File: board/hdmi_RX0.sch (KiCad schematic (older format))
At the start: 21 parts

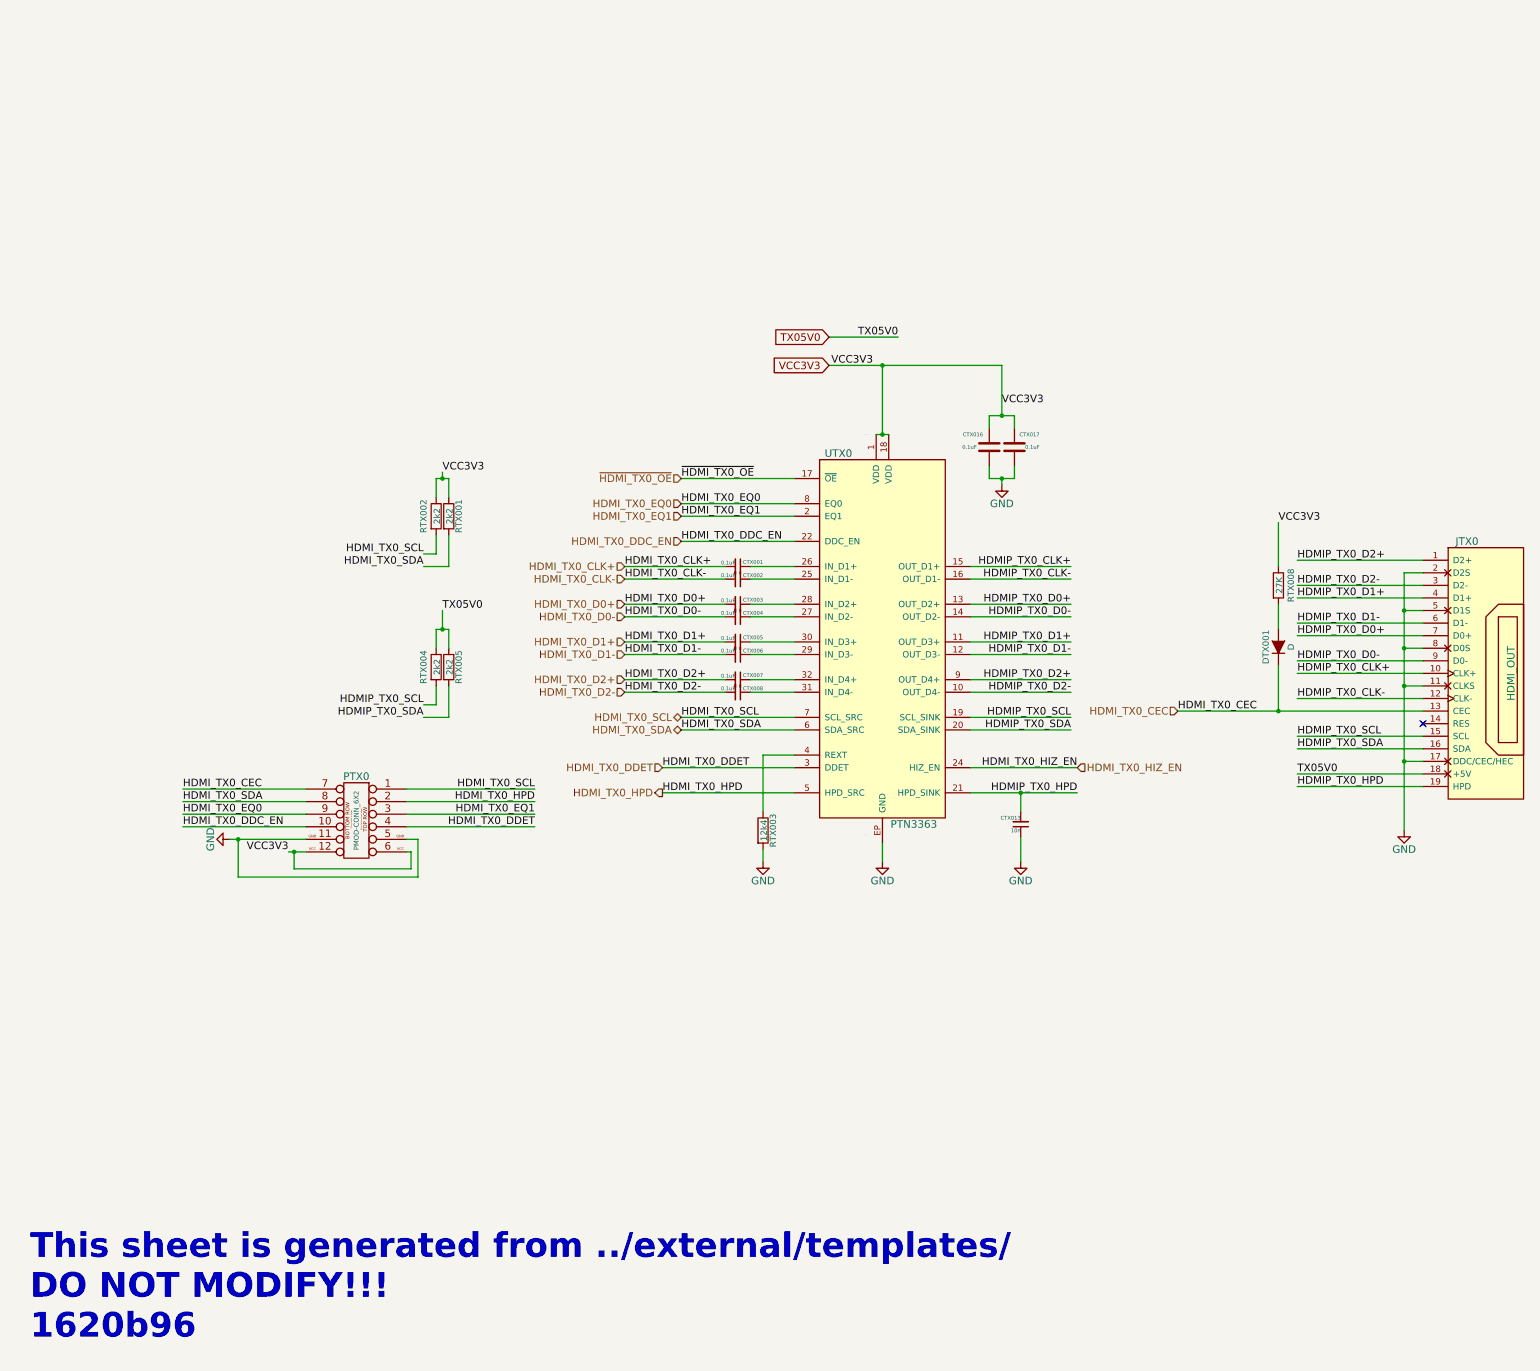
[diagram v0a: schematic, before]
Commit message: Updating from template.
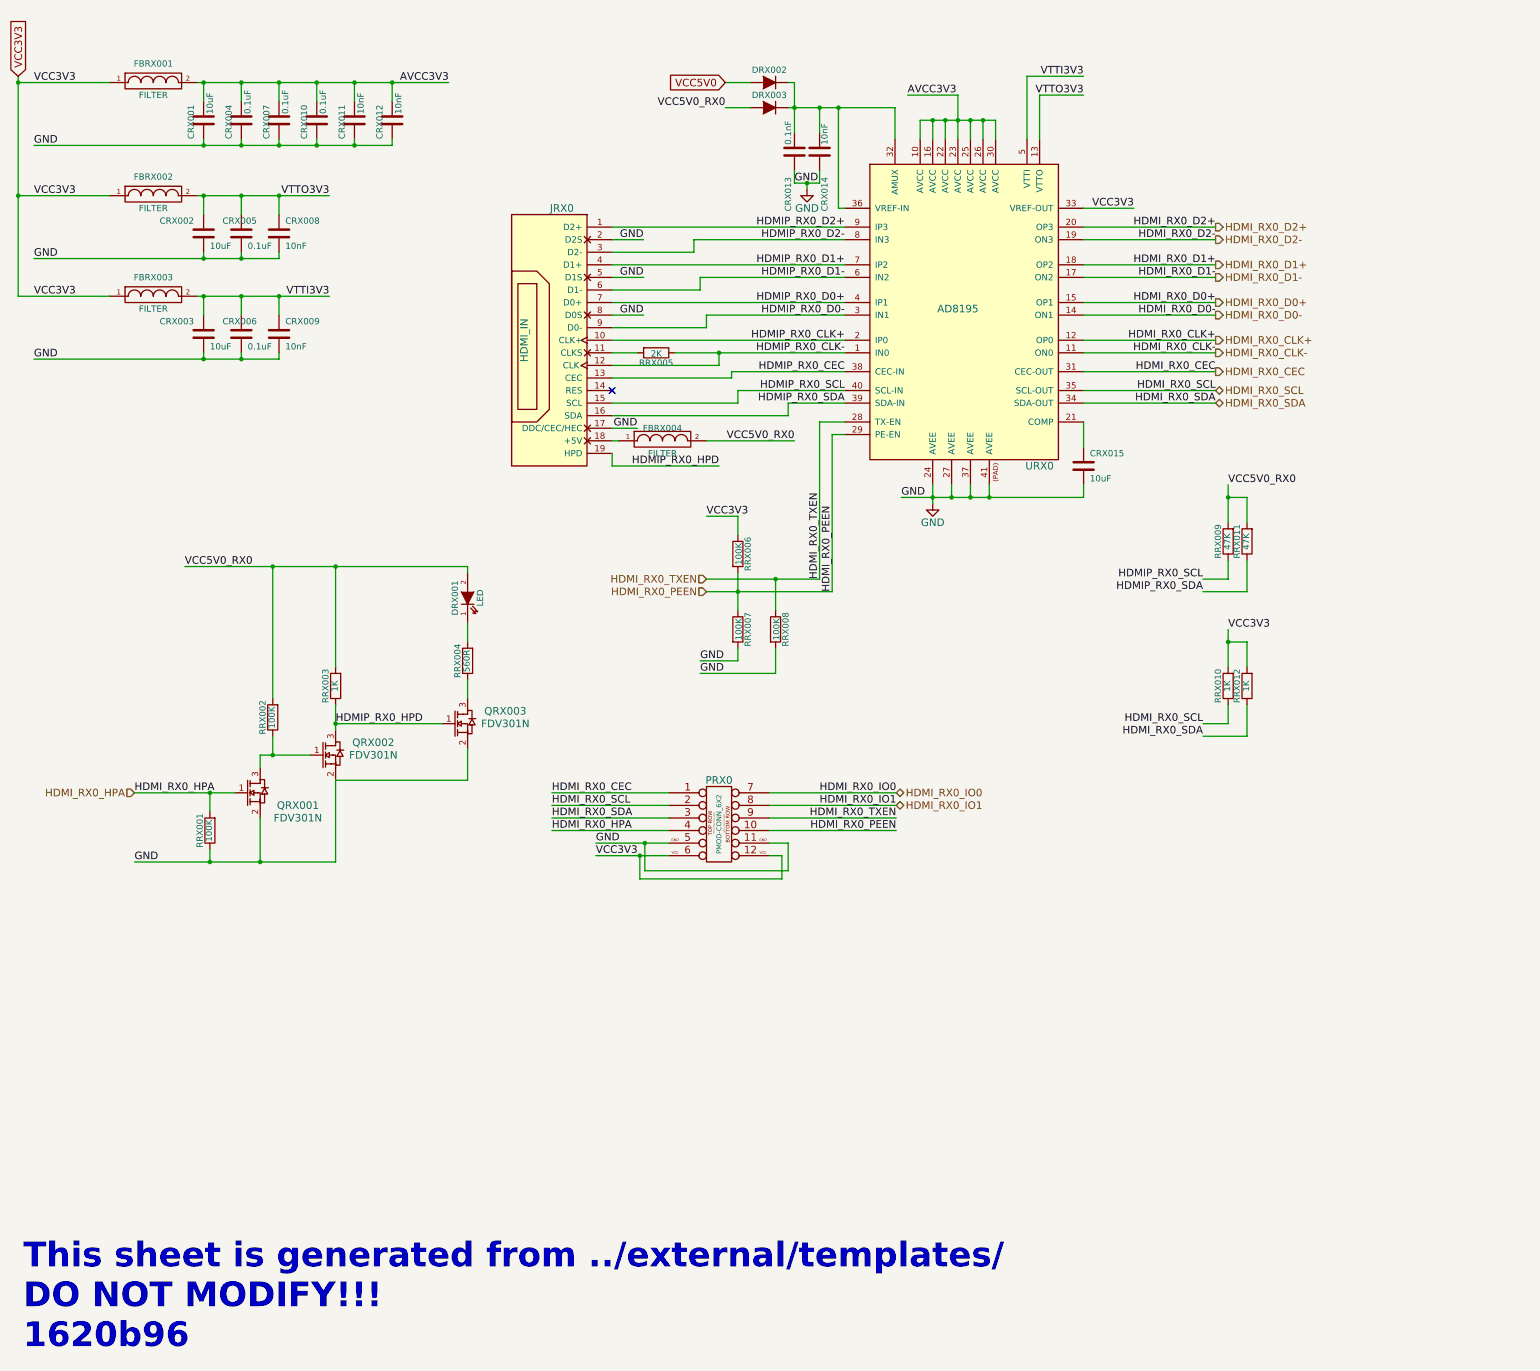
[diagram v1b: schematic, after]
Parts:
- removed CTX001, CTX002, CTX003, CTX004, CTX005, CTX006, CTX007, CTX008: 0.1uF, Capacitors_SMD:C_0402, symbol C_Small
- removed CTX013: 10n, Capacitors_SMD:C_0402, symbol C_Small
- removed CTX016, CTX017: 0.1uF, Capacitors_SMD:C_0402, symbol C
- removed DTX001: D, Diodes_SMD:SOD-523, symbol D
- removed JTX0: HDMI_OUT, hdmi:HDMI_TH, symbol HDMI_OUT
- removed PTX0: PMOD-CONN_6X2, pmod:pmod_pin_array_6x2, symbol PMOD-CONN_6X2
- removed RTX001, RTX002, RTX004, RTX005: 2k2, Resistors_SMD:R_0402, symbol R
- removed RTX003: 12k4, Resistors_SMD:R_0402, symbol R
- removed RTX008: 27K, Resistors_SMD:R_0402, symbol R
- removed UTX0: PTN3363, Housings_DFN_QFN:QFN-32-1EP_5x5mm_Pitch0.5mm, symbol PTN3363
- added CRX001, CRX002, CRX003: 10uF, Capacitors_SMD:C_0603, symbol C
- added CRX004, CRX005, CRX006, CRX007, CRX010: 0.1uF, Capacitors_SMD:C_0402, symbol C
- added CRX008, CRX009, CRX011, CRX012, CRX014: 10nF, Capacitors_SMD:C_0402, symbol C
- added CRX013: 0.1nF, Capacitors_SMD:C_0402, symbol C
- added CRX015: 10uF, Capacitors_SMD:C_0402, symbol C
- added DRX001: LED, LEDs:LED_0603, symbol LED
- added DRX002, DRX003: D, Diodes_SMD:SOD-123, symbol D
- added FBRX001, FBRX002, FBRX003, FBRX004: FILTER, Capacitors_SMD:C_0805, symbol FILTER
- added JRX0: HDMI_IN, hdmi:HDMI_TH, symbol HDMI_IN
- added PRX0: PMOD-CONN_6X2, pmod:pmod_pin_array_6x2, symbol PMOD-CONN_6X2
- added QRX001, QRX002, QRX003: FDV301N, TO_SOT_Packages_SMD:SOT-23, symbol FDV301N
- added RRX001, RRX002, RRX006, RRX007, RRX008: 100K, Resistors_SMD:R_0402, symbol R
- added RRX003, RRX010, RRX012: 1K, Resistors_SMD:R_0402, symbol R
- added RRX004: 560R, Resistors_SMD:R_0402, symbol R
- added RRX005: 2K, Resistors_SMD:R_0402, symbol R
- added RRX009, RRX011: 47K, Resistors_SMD:R_0402, symbol R
- added URX0: AD8195, Housings_DFN_QFN:QFN-40-1EP_6x6mm_Pitch0.5mm, symbol AD8195
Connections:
- net GND: now also CRX001.2, CRX002.2, CRX003.2, CRX004.2, CRX005.2, CRX006.2, CRX007.2, CRX008.2, CRX009.2, CRX010.2, CRX011.2, CRX012.2, CRX013.2, CRX014.2, CRX015.2, JRX0.17 (DDC/CEC/HEC), JRX0.2 (D2S), JRX0.5 (D1S), JRX0.8 (D0S), PRX0.11 (P11), PRX0.5 (P5), QRX001.2, QRX002.2, QRX003.2, RRX001.1, RRX007.2, RRX008.2, URX0.24 (AVEE), URX0.27 (AVEE), URX0.37 (AVEE), URX0.41 (AVEE)
- net VCC3V3: now also FBRX001.1, FBRX002.1, FBRX003.1, PRX0.12 (P12), PRX0.6 (P6), RRX006.1, RRX010.2, RRX012.2, URX0.33 (VREF-OUT)
- new net: CRX015.1, URX0.21 (COMP)
- new net: CRX013.1, CRX014.1, DRX002.1 (K), DRX003.1 (K), URX0.32 (AMUX), URX0.36 (VREF-IN)
- new net: JRX0.11 (CLKS), RRX005.2
- new net: FBRX004.1, JRX0.18 (+5V)
- new net: QRX001.3, QRX002.1, RRX002.1
- new net: QRX003.3, RRX004.1
- new net: DRX001.1 (K), RRX004.2
- new net AVCC3V3: CRX001.1, CRX004.1, CRX007.1, CRX010.1, CRX011.1, CRX012.1, FBRX001.2, URX0.10 (AVCC), URX0.16 (AVCC), URX0.22 (AVCC), URX0.23 (AVCC), URX0.25 (AVCC), URX0.26 (AVCC), URX0.30 (AVCC)
- new net HDMIP_RX0_CEC: JRX0.13 (CEC), URX0.38 (CEC-IN)
- new net HDMIP_RX0_CLK+: JRX0.10 (CLK+), URX0.2 (IP0)
- new net HDMIP_RX0_CLK-: JRX0.12 (CLK-), RRX005.1, URX0.1 (IN0)
- new net HDMIP_RX0_D0+: JRX0.7 (D0+), URX0.4 (IP1)
- new net HDMIP_RX0_D0-: JRX0.9 (D0-), URX0.3 (IN1)
- new net HDMIP_RX0_D1+: JRX0.4 (D1+), URX0.7 (IP2)
- new net HDMIP_RX0_D1-: JRX0.6 (D1-), URX0.6 (IN2)
- new net HDMIP_RX0_D2+: JRX0.1 (D2+), URX0.9 (IP3)
- new net HDMIP_RX0_D2-: JRX0.3 (D2-), URX0.8 (IN3)
- new net HDMIP_RX0_HPD: JRX0.19 (HPD), QRX002.3, QRX003.1, RRX003.1
- new net HDMIP_RX0_SCL: JRX0.15 (SCL), RRX009.1, URX0.40 (SCL-IN)
- new net HDMIP_RX0_SDA: JRX0.16 (SDA), RRX011.1, URX0.39 (SDA-IN)
- new net HDMI_RX0_CEC: PRX0.1 (P1), URX0.31 (CEC-OUT)
- new net HDMI_RX0_CLK+: URX0.12 (OP0)
- new net HDMI_RX0_CLK-: URX0.11 (ON0)
- new net HDMI_RX0_D0+: URX0.15 (OP1)
- new net HDMI_RX0_D0-: URX0.14 (ON1)
- new net HDMI_RX0_D1+: URX0.18 (OP2)
- new net HDMI_RX0_D1-: URX0.17 (ON2)
- new net HDMI_RX0_D2+: URX0.20 (OP3)
- new net HDMI_RX0_D2-: URX0.19 (ON3)
- new net HDMI_RX0_HPA: PRX0.4 (P4), QRX001.1, RRX001.2
- new net HDMI_RX0_IO0: PRX0.7 (P7)
- new net HDMI_RX0_IO1: PRX0.8 (P8)
- new net HDMI_RX0_PEEN: PRX0.10 (P10), RRX006.2, RRX007.1, URX0.29 (PE-EN)
- new net HDMI_RX0_SCL: PRX0.2 (P2), RRX010.1, URX0.35 (SCL-OUT)
- new net HDMI_RX0_SDA: PRX0.3 (P3), RRX012.1, URX0.34 (SDA-OUT)
- new net HDMI_RX0_TXEN: PRX0.9 (P9), RRX008.1, URX0.28 (TX-EN)
- new net VCC5V0: DRX002.2 (A)
- new net VCC5V0_RX0: DRX001.2 (A), DRX003.2 (A), FBRX004.2, RRX002.2, RRX003.2, RRX009.2, RRX011.2
- new net VTTI3V3: CRX003.1, CRX006.1, CRX009.1, FBRX003.2, URX0.5 (VTTI)
- new net VTTO3V3: CRX002.1, CRX005.1, CRX008.1, FBRX002.2, URX0.13 (VTTO)
